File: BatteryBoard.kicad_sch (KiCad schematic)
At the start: 4 parts

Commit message: Updated version to v2.1
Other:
- company: (none) -> Carnegie Mellon University
- title: (none) -> Argus Batteryboard
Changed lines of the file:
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@@
 	(generator_version "8.0")
 	(paper "A4")
+	(title_block
+		(title "Argus Batteryboard")
+		(date "2024-11-19")
+		(rev "v2.1")
+		(company "Carnegie Mellon University")
+		(comment 1 "M. Holliday")
+		(comment 2 "N. Khera")
+		(comment 3 "V. Rajesh")
+	)
 	(junction
 		(at 200.66 121.92)

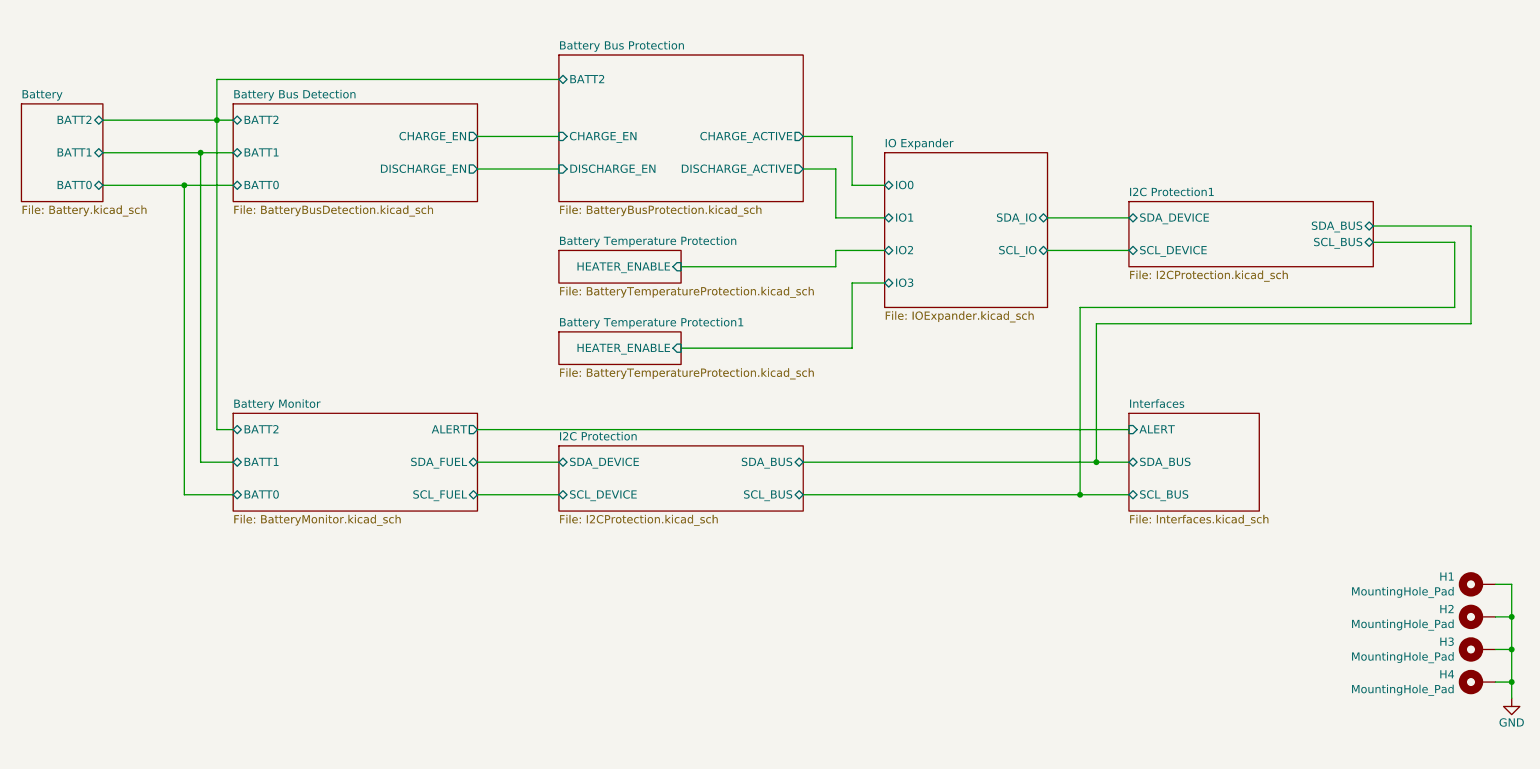
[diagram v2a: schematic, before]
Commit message: v2.1 (v3?) Partial Updates
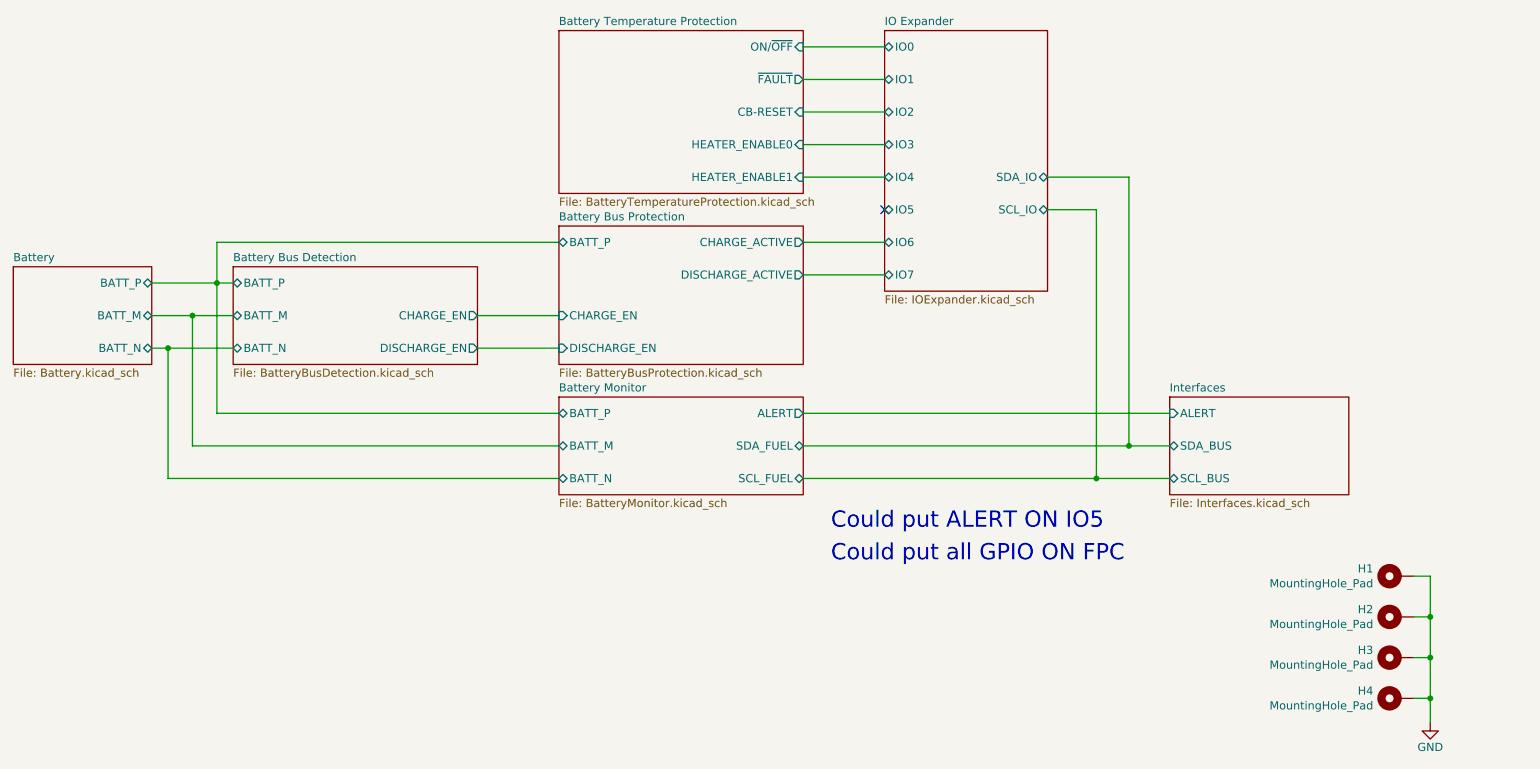
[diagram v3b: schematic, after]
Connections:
- no-connect marks 0 -> 1
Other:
- removed sheet Battery Temperature Protection1
- removed sheet I2C Protection
- removed sheet I2C Protection1
- sheet Battery ports: added BATT_M, BATT_N, BATT_P; removed BATT0, BATT1, BATT2
- sheet Battery Bus Detection ports: added BATT_M, BATT_N, BATT_P; removed BATT0, BATT1, BATT2
- sheet Battery Bus Protection ports: added BATT_P; removed BATT2
- sheet Battery Monitor ports: added BATT_M, BATT_N, BATT_P; removed BATT0, BATT1, BATT2
- sheet Battery Temperature Protection ports: added CB-RESET, HEATER_ENABLE0, HEATER_ENABLE1, ON/~{OFF}, ~{FAULT}; removed HEATER_ENABLE
- sheet IO Expander ports: added IO4, IO5, IO6, IO7; removed none
- note added: "Could put ALERT ON IO5"
- note added: "Could put all GPIO ON FPC"
- moved on the sheet: H1, H2, H3, H4
